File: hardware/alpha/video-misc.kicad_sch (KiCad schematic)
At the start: 21 parts, among them U1 L78L05_SO8, U3 L79L05_SO8, U6 TLE2082, U8 MCP47FEB22A0-E/ST

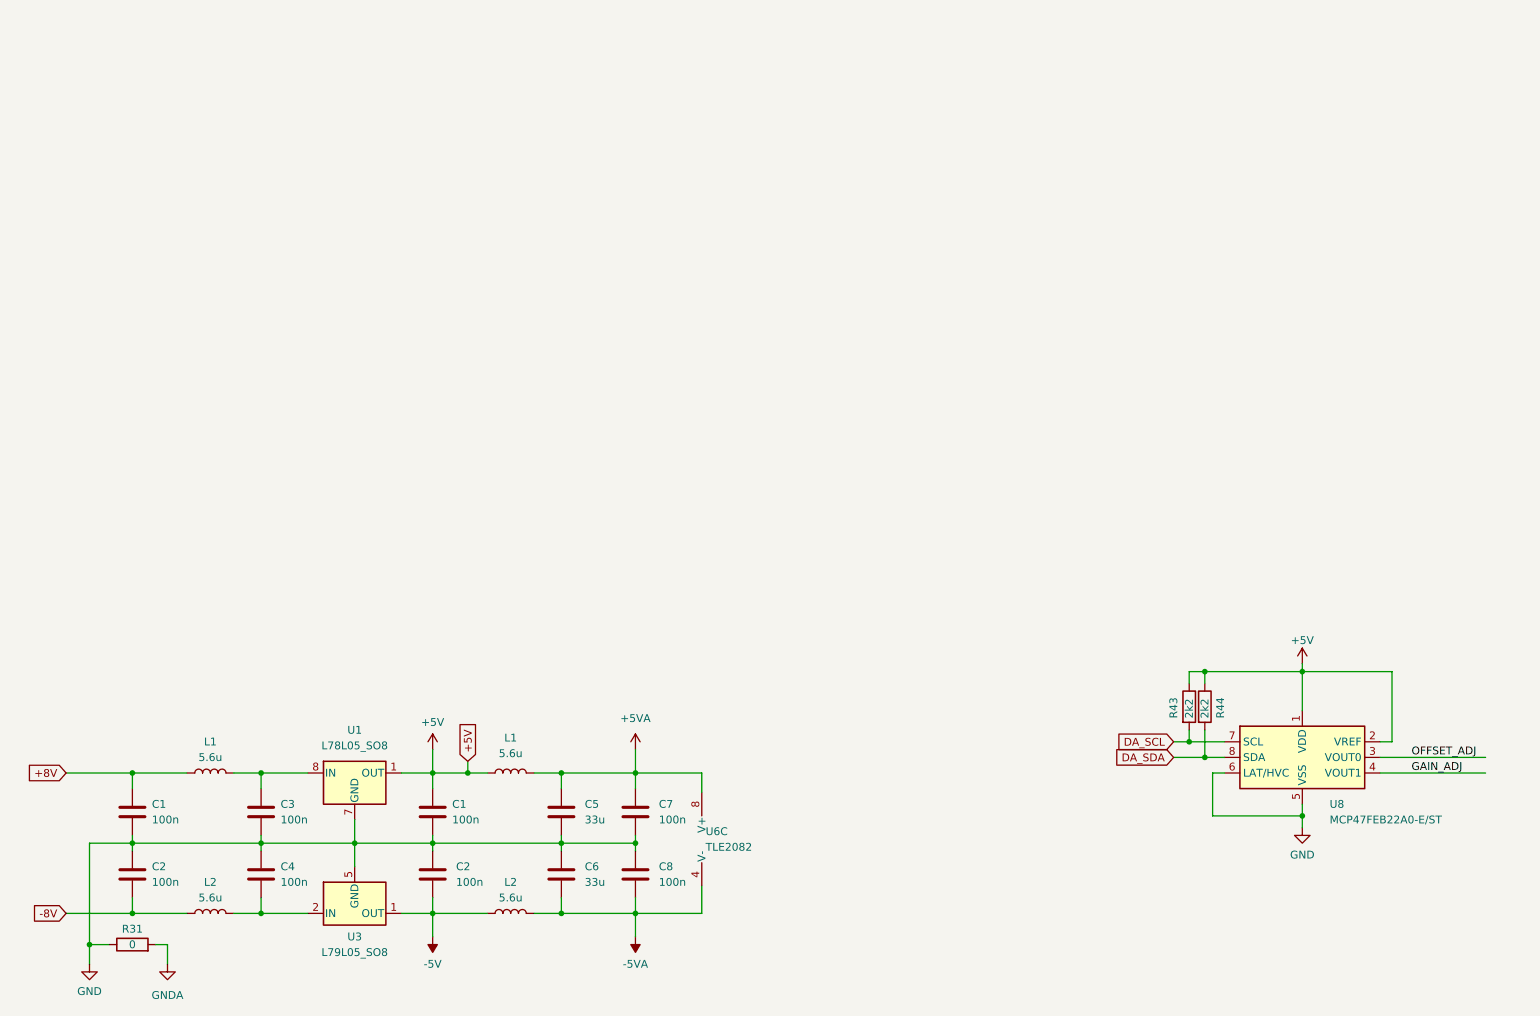
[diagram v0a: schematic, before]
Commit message: WIP
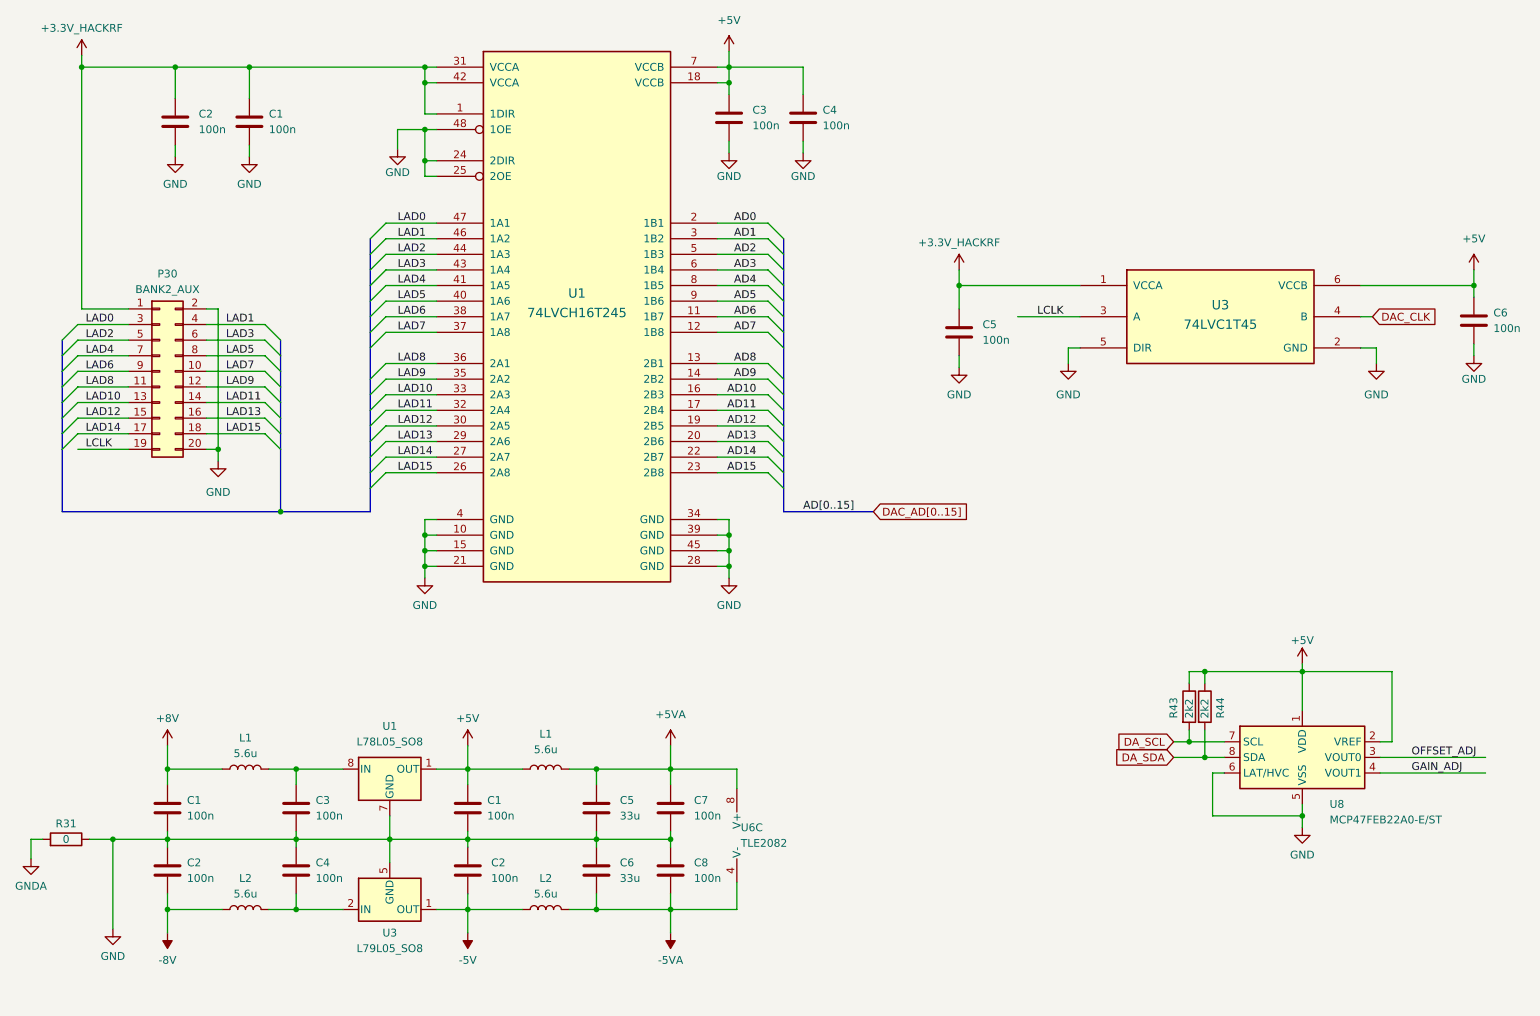
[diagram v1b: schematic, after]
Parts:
- added C1, C2, C3, C4, C5, C6: 100n, symbol Device:C
- added P30: BANK2_AUX, symbol Connector_Generic:Conn_02x10_Odd_Even
- added U1: 74LVCH16T245, symbol 74lvc16t245:74LVC16T245
- added U3: 74LVC1T45, symbol 74lvc1t45:74LVC1T45
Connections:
- net +5V: now also C3.1, C4.1, C6.1, U1.18 (VCCB), U1.7 (VCCB), U3.6 (VCCB)
- net GND: now also C1.2, C2.2, C3.2, C4.2, C5.2, C6.2, P30.2 (Pin_2), P30.20 (Pin_20), U1.10 (GND), U1.15 (GND), U1.21 (GND), U1.24 (2DIR), U1.25 (2OE), U1.28 (GND), U1.34 (GND), U1.39 (GND), U1.4 (GND), U1.45 (GND), U1.48 (1OE), U3.2 (GND), U3.5 (DIR)
- new net +3.3VP: C1.1, C2.1, C5.1, P30.1 (Pin_1), U1.1 (1DIR), U1.31 (VCCA), U1.42 (VCCA), U3.1 (VCCA)
- new net AD0: U1.2 (1B1)
- new net AD1: U1.3 (1B2)
- new net AD10: U1.16 (2B3)
- new net AD11: U1.17 (2B4)
- new net AD12: U1.19 (2B5)
- new net AD13: U1.20 (2B6)
- new net AD14: U1.22 (2B7)
- new net AD15: U1.23 (2B8)
- new net AD2: U1.5 (1B3)
- new net AD3: U1.6 (1B4)
- new net AD4: U1.8 (1B5)
- new net AD5: U1.9 (1B6)
- new net AD6: U1.11 (1B7)
- new net AD7: U1.12 (1B8)
- new net AD8: U1.13 (2B1)
- new net AD9: U1.14 (2B2)
- new net DAC_CLK: U3.4 (B)
- new net LAD0: P30.3 (Pin_3), U1.47 (1A1)
- new net LAD1: P30.4 (Pin_4), U1.46 (1A2)
- new net LAD10: P30.13 (Pin_13), U1.33 (2A3)
- new net LAD11: P30.14 (Pin_14), U1.32 (2A4)
- new net LAD12: P30.15 (Pin_15), U1.30 (2A5)
- new net LAD13: P30.16 (Pin_16), U1.29 (2A6)
- new net LAD14: P30.17 (Pin_17), U1.27 (2A7)
- new net LAD15: P30.18 (Pin_18), U1.26 (2A8)
- new net LAD2: P30.5 (Pin_5), U1.44 (1A3)
- new net LAD3: P30.6 (Pin_6), U1.43 (1A4)
- new net LAD4: P30.7 (Pin_7), U1.41 (1A5)
- new net LAD5: P30.8 (Pin_8), U1.40 (1A6)
- new net LAD6: P30.9 (Pin_9), U1.38 (1A7)
- new net LAD7: P30.10 (Pin_10), U1.37 (1A8)
- new net LAD8: P30.11 (Pin_11), U1.36 (2A1)
- new net LAD9: P30.12 (Pin_12), U1.35 (2A2)
- new net LCLK: P30.19 (Pin_19), U3.3 (A)
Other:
- moved on the sheet: C1, C2, C3, C4, C5, C6, C7, C8, L1, L2, R31, U1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

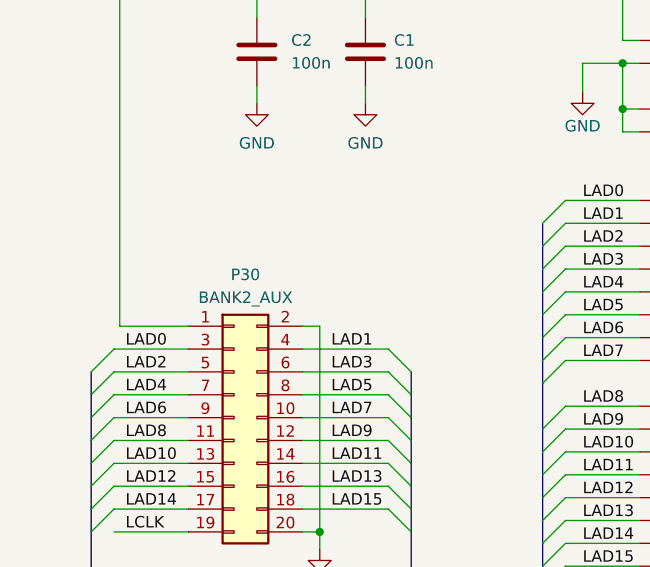
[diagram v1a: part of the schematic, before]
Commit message: WIP
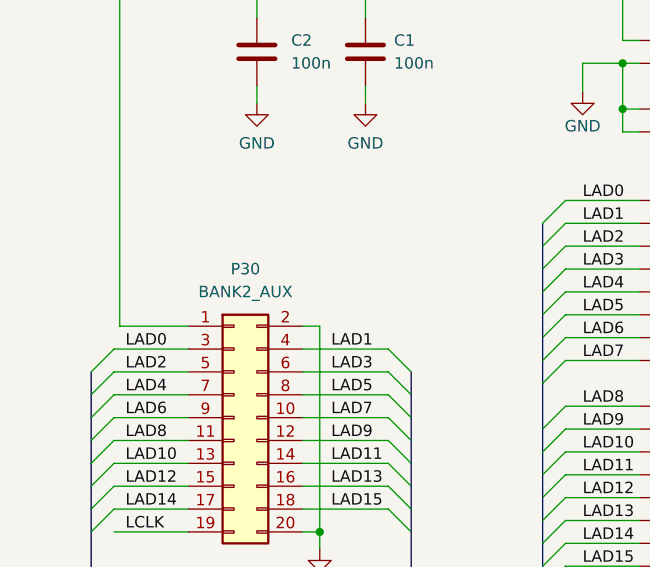
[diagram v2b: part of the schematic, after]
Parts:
- C1, C2, C3, C4, C5, C6: footprint (none) -> Capacitor_SMD:C_0603_1608Metric
- P30: footprint (none) -> hackrf:GSG-HEADER-2x10
- U1: footprint (none) -> Package_TO_SOT_SMD:SOT-23-6
- U3: footprint (none) -> Package_SO:TSSOP-48_6.1x12.5mm_P0.5mm
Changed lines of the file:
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@@
       (effects (font (size 1.27 1.27)) (justify left))
     )
-    (property "Footprint" "" (at 144.4752 41.275 0)
+    (property "Footprint" "Capacitor_SMD:C_0603_1608Metric" (at 144.4752 41.275 0)
       (effects (font (size 1.27 1.27)) hide)
     )
@@
       (effects (font (size 1.27 1.27)) (justify left))
     )
-    (property "Footprint" "" (at 181.9402 76.2 0)
+    (property "Footprint" "Capacitor_SMD:C_0603_1608Metric" (at 181.9402 76.2 0)
       (effects (font (size 1.27 1.27)) hide)
     )
@@
       (effects (font (size 1.27 1.27)) (justify left))
     )
-    (property "Footprint" "" (at 156.5402 41.275 0)
+    (property "Footprint" "Capacitor_SMD:C_0603_1608Metric" (at 156.5402 41.275 0)
       (effects (font (size 1.27 1.27)) hide)
     )
@@
       (effects (font (size 1.27 1.27)) (justify left))
     )
-    (property "Footprint" "" (at 54.3052 41.91 0)
+    (property "Footprint" "Capacitor_SMD:C_0603_1608Metric" (at 54.3052 41.91 0)
       (effects (font (size 1.27 1.27)) hide)
     )
@@
       (effects (font (size 1.524 1.524)))
     )
-    (property "Footprint" "" (at 118.745 68.58 0)
+    (property "Footprint" "Package_TO_SOT_SMD:SOT-23-6" (at 118.745 68.58 0)
       (effects (font (size 1.27 1.27)) hide)
     )
@@
       (effects (font (size 1.524 1.524)))
     )
-    (property "Footprint" "" (at 222.25 69.85 0)
+    (property "Footprint" "Package_SO:TSSOP-48_6.1x12.5mm_P0.5mm" (at 222.25 69.85 0)
       (effects (font (size 1.27 1.27)) hide)
     )
@@
   (symbol (lib_id "Connector_Generic:Conn_02x10_Odd_Even") (at 50.8 78.74 0) (unit 1)
     (in_bom yes) (on_board yes) (dnp no) (fields_autoplaced)
-    (property "Reference" "P30" (at 52.07 62.865 0)
-      (effects (font (size 1.27 1.27)))
-    )
-    (property "Value" "BANK2_AUX" (at 52.07 65.405 0)
-      (effects (font (size 1.27 1.27)))
-    )
-    (property "Footprint" "" (at 50.8 78.74 0)
+    (property "Reference" "P30" (at 52.07 62.23 0)
+      (effects (font (size 1.27 1.27)))
+    )
+    (property "Value" "BANK2_AUX" (at 52.07 64.77 0)
+      (effects (font (size 1.27 1.27)))
+    )
+    (property "Footprint" "hackrf:GSG-HEADER-2x10" (at 50.8 78.74 0)
       (effects (font (size 1.27 1.27)) hide)
     )
@@
         )
         (path "/487245ca-0c1f-4f9d-bc99-20c8f558090f/e1e307fe-d49b-45b6-b177-774a7a482979"
-          (reference "P1") (unit 1)
+          (reference "P30") (unit 1)
         )
       )
@@
       (effects (font (size 1.27 1.27)) (justify left))
     )
-    (property "Footprint" "" (at 265.7602 74.295 0)
+    (property "Footprint" "Capacitor_SMD:C_0603_1608Metric" (at 265.7602 74.295 0)
       (effects (font (size 1.27 1.27)) hide)
     )
@@
       (effects (font (size 1.27 1.27)) (justify left))
     )
-    (property "Footprint" "" (at 66.3702 41.91 0)
-      (effects (font (size 1.27 1.27)) hide)
-    )
+    (property "Footprint" "Capacitor_SMD:C_0603_1608Metric" (at 66.3702 41.91 0)
+      (effects (font (size 1.27 1.27)) hide)
+    )
